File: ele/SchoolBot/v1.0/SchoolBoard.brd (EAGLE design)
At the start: 95 x 60 mm, 55 parts, among them X1 M8, X2 M8, X4 POWER_IN

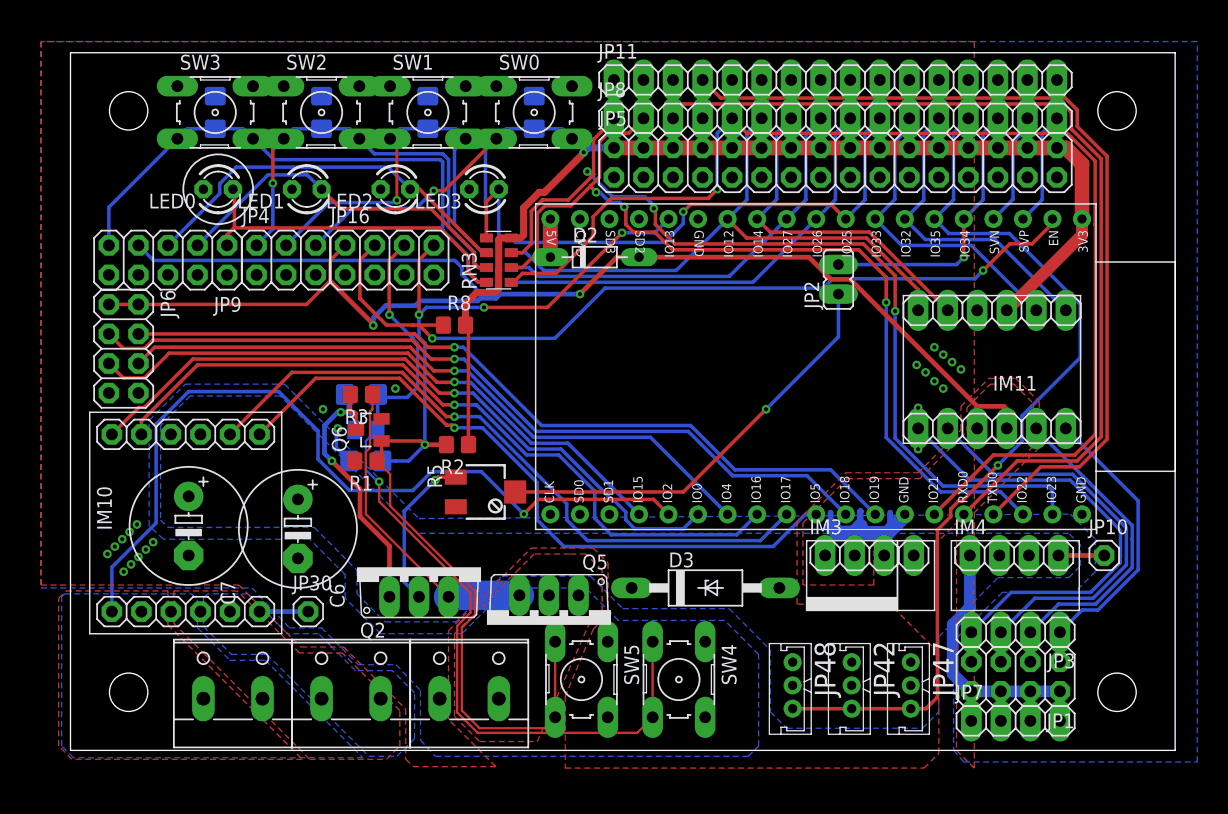
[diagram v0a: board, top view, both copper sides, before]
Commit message: RB3202_jednotny_konektor_na_motory
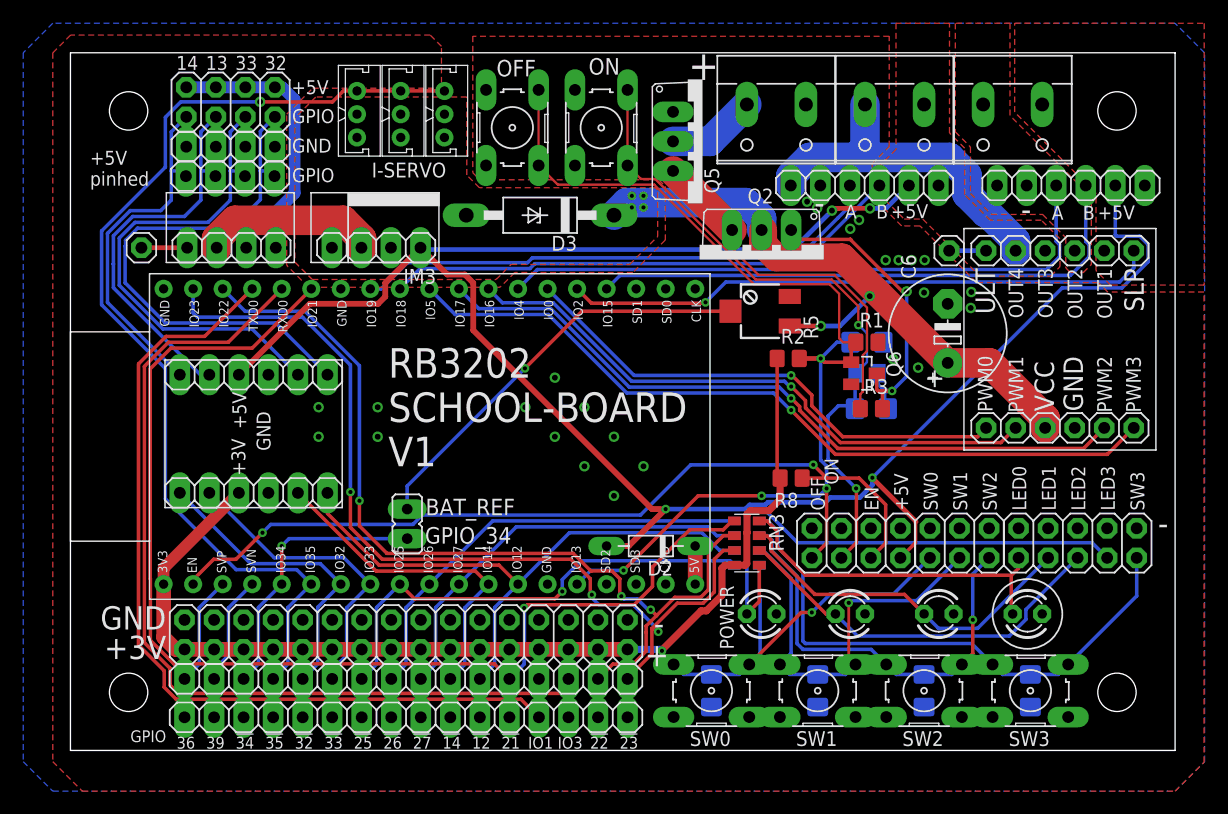
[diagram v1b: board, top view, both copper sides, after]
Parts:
- removed C7: (no value), rcl:E5-10,5
- added JP12: (no value), pinhead:1X06
- JP6: device pinhead:2X04 -> pinhead:1X06
- moved JP10 86.9 mm to (6.10, 43.2), turned to 180 degrees
- moved C8 86.0 mm to (82.5, 5.13), turned to 90 degrees
- moved SW3 86.0 mm to (82.5, 5.13), turned to 180 degrees
- moved JP1 83.7 mm to (13.8, 55.8), turned to 0 degrees
- moved JP7 83.6 mm to (13.8, 51.9), turned to 180 degrees
- moved X1 83.5 mm to (81.0, 54.9), turned to 180 degrees
- moved JP9 81.9 mm to (86.6, 17.8), turned to 0 degrees
- moved IM11 80.8 mm to (8.13, 20.9), turned to 0 degrees
- moved LED0 78.6 mm to (82.3, 11.7), turned to 0 degrees
- moved JP3 78.1 mm to (13.7, 49.4), turned to 0 degrees
- moved C4 71.8 mm to (73.4, 5.13), turned to 90 degrees
- moved SW2 71.8 mm to (73.4, 5.13), turned to 180 degrees
- moved IM10 68.7 mm to (77.5, 44.2), turned to 270 degrees
- moved JP47 68.4 mm to (24.6, 54.7), turned to 90 degrees
- moved X2 68.3 mm to (70.9, 54.9), turned to 180 degrees
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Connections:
- net +5V: now also JP12.5; no longer JP6.1
- net ENC_A1: now also JP12.3; no longer JP6.6
- net ENC_A2: now also IM6.31, JP6.4; no longer IM6.30, JP6.3
- net ENC_B1: now also IM6.23, JP12.4; no longer IM6.31, JP6.4
- net ENC_B2: now also IM6.30, JP6.3; no longer IM6.23, JP6.5
- net GND: now also JP12.2, JP6.5; no longer C7.-, JP6.7, JP6.8
- net M1A: now also JP12.6
- net M1B: now also JP12.1
- net M2A: now also JP6.1
- net M2B: now also JP6.6
- net PWM0: now also IM6.25; no longer IM6.29
- net PWM1: now also IM6.27; no longer IM6.28
- net PWM2: now also IM6.28; no longer IM6.27
- net PWM3: now also IM6.29; no longer IM6.25
- net VCC: no longer C7.+
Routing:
- net +5V: track 93.3 -> 172.9 mm, vias 2 -> 4
- net VCC: track 13.5 -> 71.4 mm, vias 1 -> 6
- net M2B: track 0.00 -> 30.5 mm
- net ENC_A2: track 70.4 -> 46.0 mm, vias 1 -> 0
- net GND: track 22.2 -> 0.00 mm, vias 23 -> 25
- net ENC_B1: track 69.8 -> 48.9 mm, vias 1 -> 0
- net SLEEP: track 71.1 -> 51.1 mm
- net ON: track 74.3 -> 57.5 mm
- net PWM0: track 59.2 -> 43.9 mm
- net GPIO35: track 80.7 -> 90.7 mm
- net ENC_B2: track 52.8 -> 44.9 mm, vias 1 -> 0
- net BAT1: track 0.00 -> 7.67 mm
- net PWM3: track 60.1 -> 67.4 mm
- net PWM1: track 57.8 -> 51.7 mm
- net GPIO33_5V: track 37.8 -> 42.7 mm
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- added copper zone on layer 1, net M1B
- added copper zone on layer 1, net VCC
- removed copper zone on layer 1, net +5V
- removed copper zone on layer 1, net BAT1
- removed copper zone on layer 16, net M1B
- removed copper zone on layer 16, net M2B
- removed copper zone on layer 16, net VCC
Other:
- board text added: "!12"
- board text added: "!14"
- board text added: "!21"
- board text added: "!22"
- board text added: "!23"
- board text added: "!25"
- board text added: "!26"
- board text added: "!27"
- board text added: "!32"
- board text added: "!33"
- board text added: "!34"
- board text added: "!35"
- board text added: "+"
- board text added: "+3V"
- board text added: "+5V"
- board text added: "+5V pinhed"
- board text added: "-"
- board text added: "13"
- board text added: "14"
- board text added: "32"
- board text added: "33"
- board text added: "36"
- board text added: "39"
- board text added: "6-11V"
- board text added: "A"
- board text added: "B"
- board text added: "BAT_REF"
- board text added: "EN"
- board text added: "GND"
- board text added: "GPIO"
- board text added: "GPIO_34"
- board text added: "I-SERVO"
- board text added: "IO1"
- board text added: "IO3"
- board text added: "LED0"
- board text added: "LED1"
- board text added: "LED2"
- board text added: "LED3"
- board text added: "OFF"
- board text added: "ON"
- board text added: "OUT1"
- board text added: "OUT2"
- board text added: "OUT3"
- board text added: "OUT4"
- board text added: "POWER"
- board text added: "PWM0"
- board text added: "PWM1"
- board text added: "PWM2"
- board text added: "PWM3"
- board text added: "RB3202 SCHOOL-BOARD V1"
- board text added: "RB3202_SCHOOL-BOARD_V1"
- board text added: "SLP"
- board text added: "SW0"
- board text added: "SW1"
- board text added: "SW2"
- board text added: "SW3"
- board text added: "ULT"
- board text added: "VCC"
